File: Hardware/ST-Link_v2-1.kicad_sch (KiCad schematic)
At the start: 38 parts, among them J1 Conn_01x06, P1 USB_C_Plug_USB2.0, U1 STM32F103CBTx, U2 LP5907MFX-3.3, U3 SRV05-4, Y1 Crystal_Small

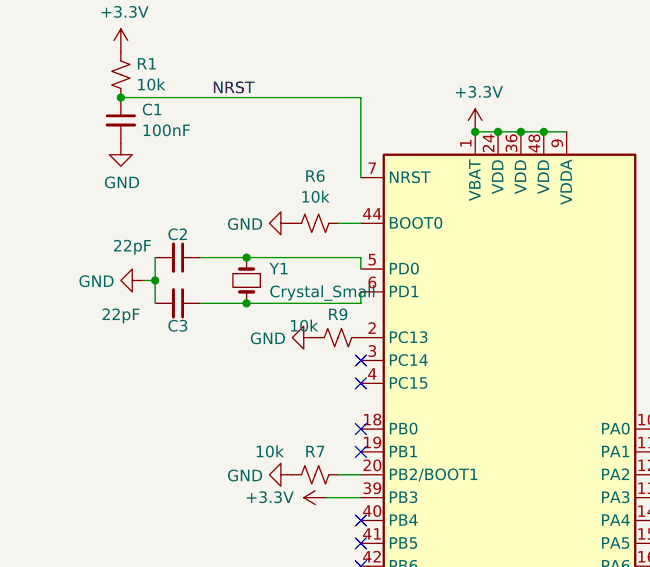
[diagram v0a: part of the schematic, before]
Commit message: v2.5
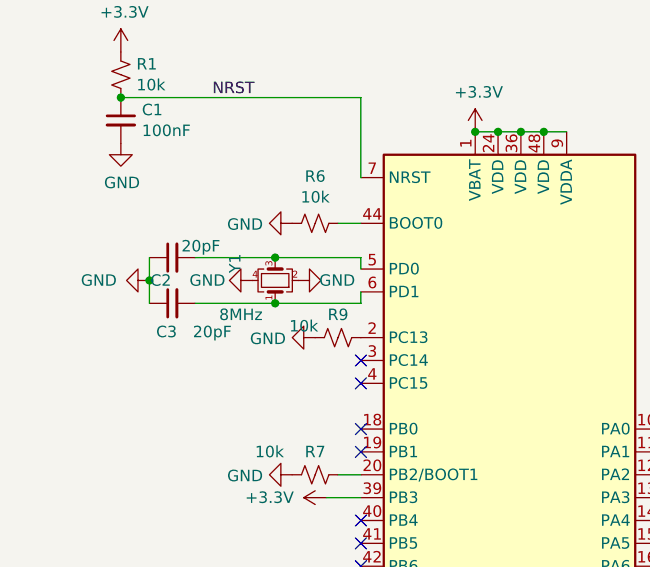
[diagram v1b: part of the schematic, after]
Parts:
- removed Y1: Crystal_Small, HKUST_RT_RCL:Crystal_HC49-4H_Vertical, symbol HKUST_RT_RCL:Crystal_Small
- added Y1: 8MHz, HKUST_RT_RCL:Crystal_SMD_3225-4Pin_3.2x2.5mm, symbol HKUST_RT_RCL:Crystal_GND24_Small
- C2, C3: value 22pF -> 20pF
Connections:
- net GND: now also C2.1, C3.1, Y1.2, Y1.4; no longer C2.2, C3.2
- net at U1.5 (PD0): now also C2.2, Y1.3; no longer C2.1
- net at U1.6 (PD1): now also C3.2, Y1.1; no longer C3.1
